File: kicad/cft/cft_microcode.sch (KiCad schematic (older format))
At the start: 20 parts, among them U1403 74AHC1G08, U1701 74AHC1G08, U1702 74HC161, U1703 74AHC1G00, U1903 SN74ACT1071

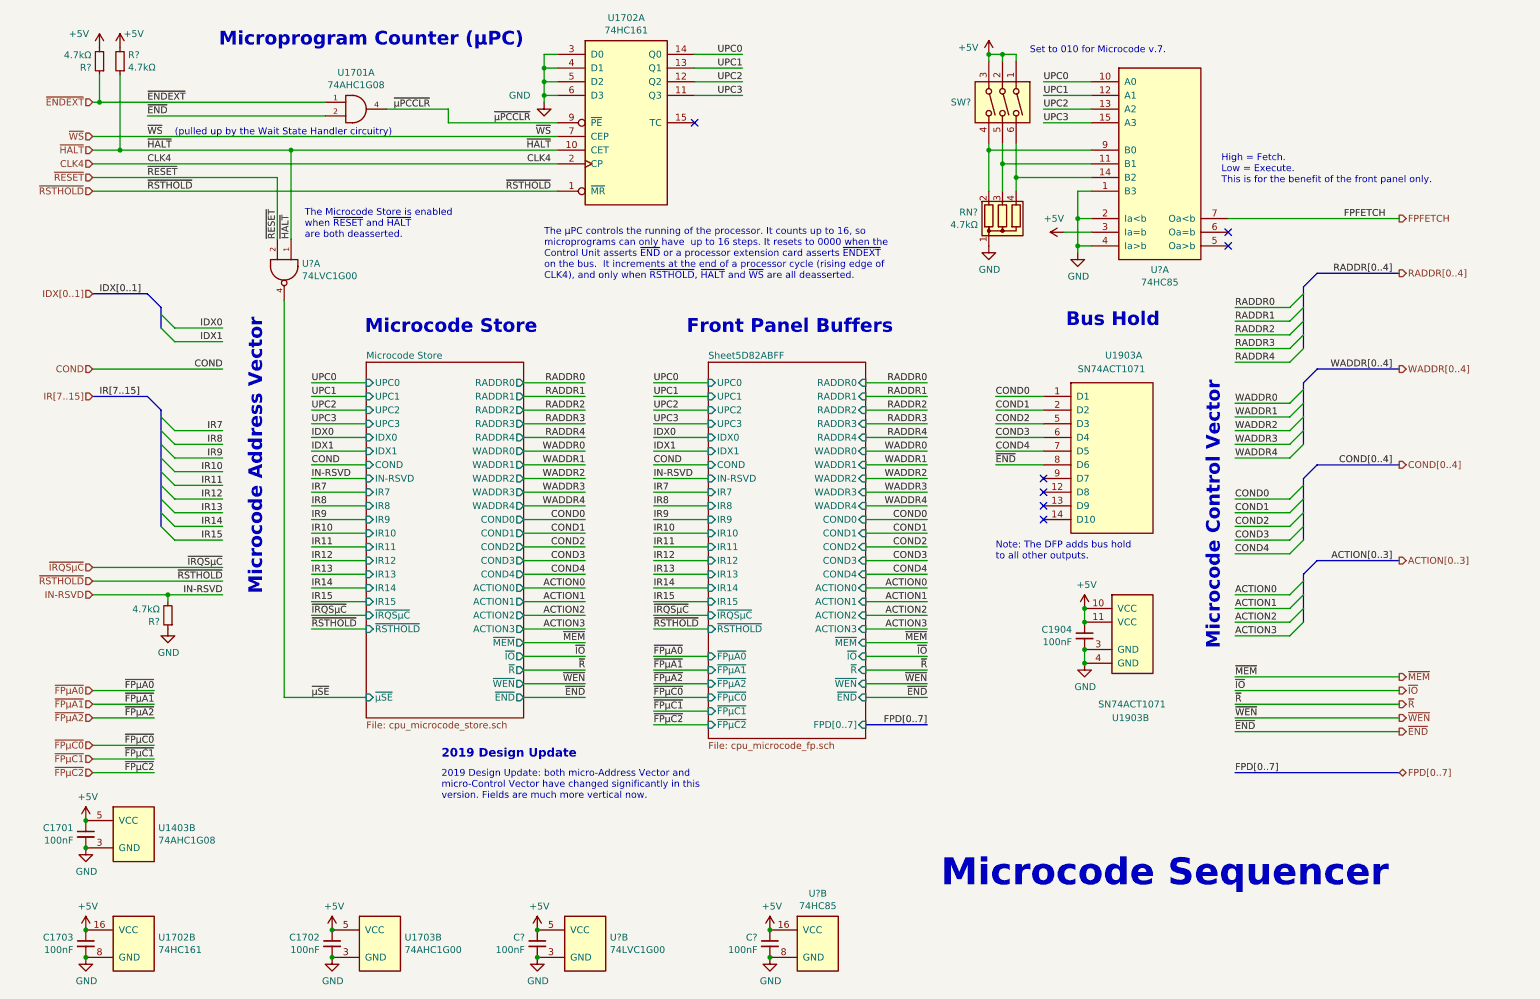
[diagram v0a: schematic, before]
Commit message: Moved things around a bit
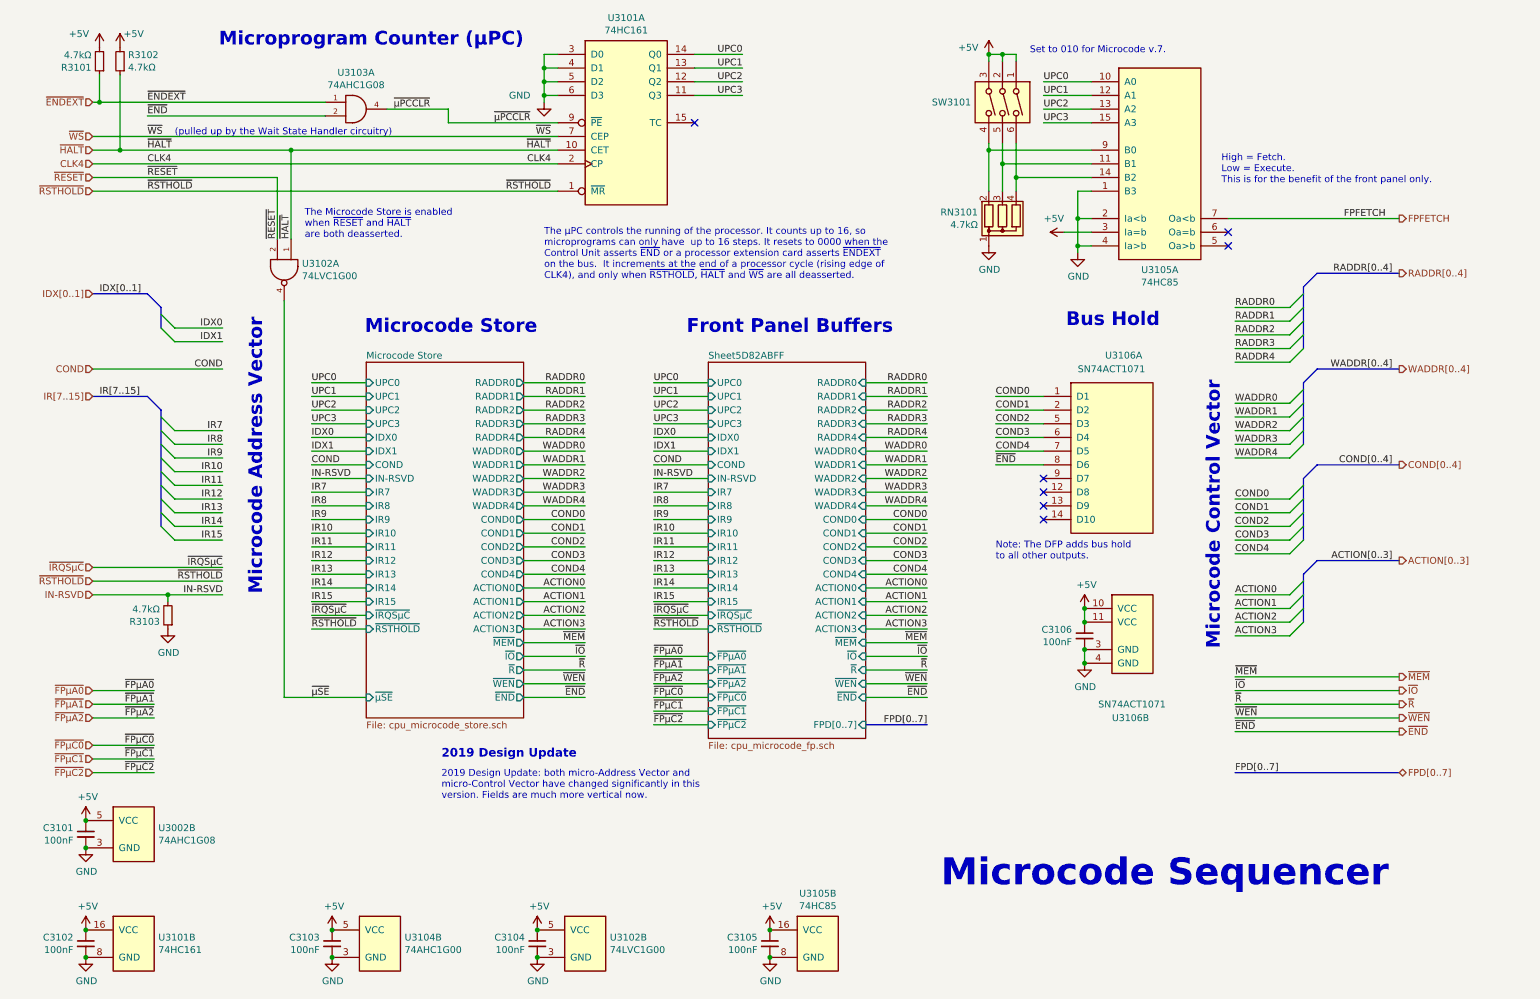
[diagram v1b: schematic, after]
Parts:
- gave numbers to parts that had none: 9
- renumbered C1701 to C3101, C1703 to C3102, C1702 to C3103, C1904 to C3106, U1403 to U3002, U1702 to U3101, U1701 to U3103, U1703 to U3104, U1903 to U3106

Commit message: Removed widebus buffer from microcode store µAddr High
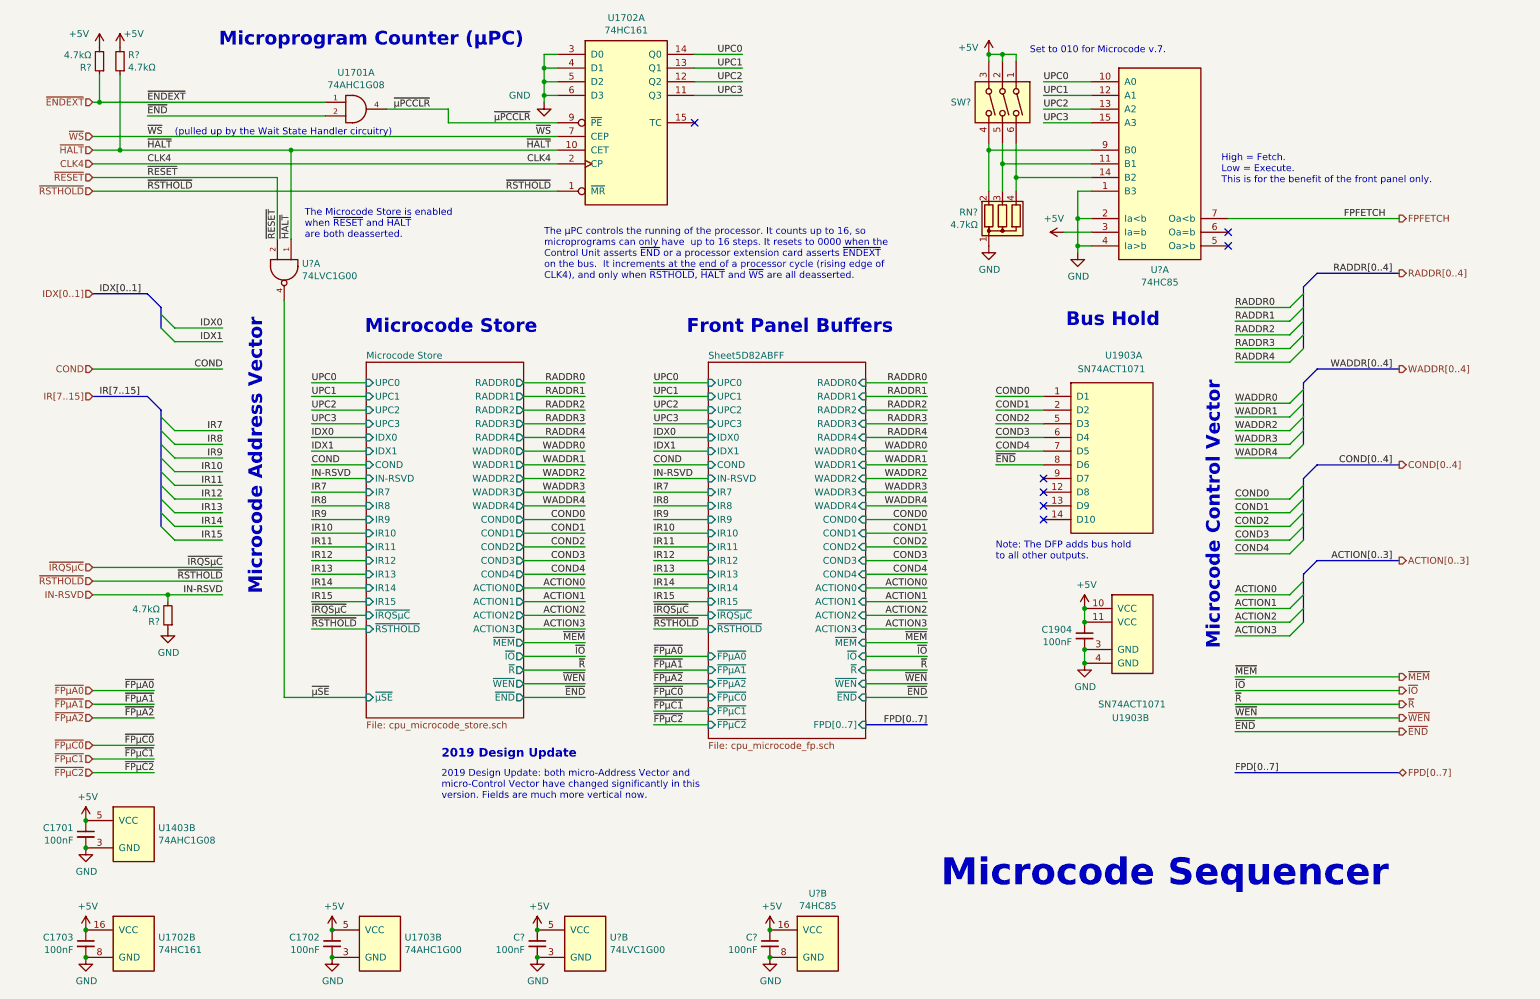
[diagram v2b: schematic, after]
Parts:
- renumbered C3101 to C1701, C3103 to C1702, C3102 to C1703, C3106 to C1904, C3104 to C?, C3105 to C?, R3103 to R?, R3101 to R?, R3102 to R?, RN3101 to RN?, SW3101 to SW?, U3002 to U1403, U3103 to U1701, U3101 to U1702, U3104 to U1703, U3106 to U1903, U3102 to U?, U3105 to U?
